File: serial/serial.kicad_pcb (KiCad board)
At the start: 2 copper layers, 24.2 x 12.2 mm, 8 parts, among them J2 Conn_02x03_Odd_Even, Q1 BSS138

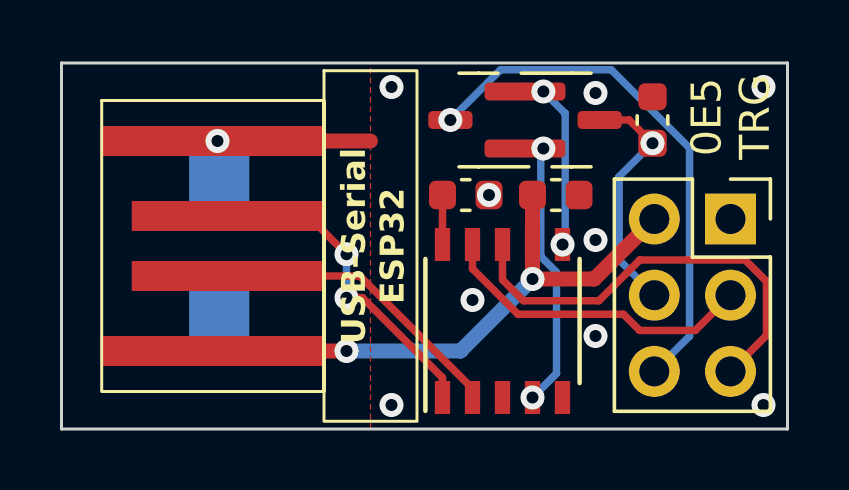
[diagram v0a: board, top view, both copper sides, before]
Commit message: -
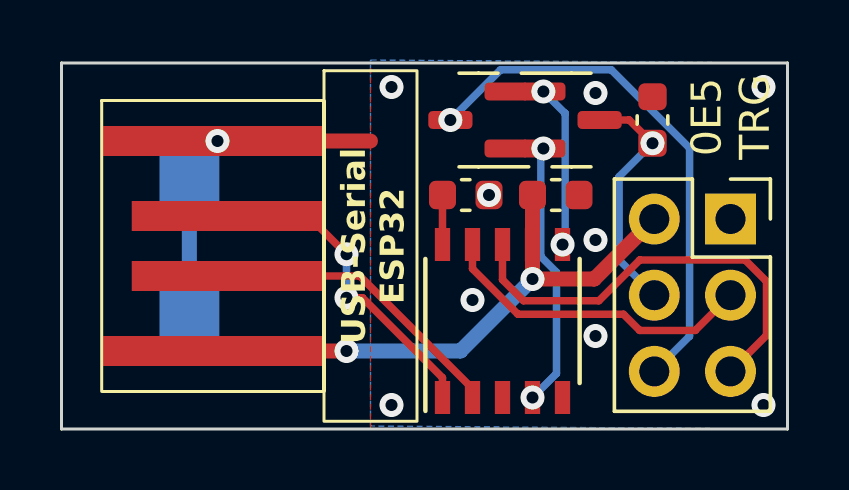
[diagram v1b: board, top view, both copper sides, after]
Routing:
- net Net-(J2-Pin_1): track 5.10 -> 10.6 mm
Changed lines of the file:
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@@
     (pad "4" smd rect (at 4.945 3.5) (size 7.41 1) (layers "F.Cu" "F.Paste" "F.Mask")
       (net 1 "Net-(J2-Pin_2)") (pinfunction "VBUS") (pintype "power_in") (thermal_bridge_angle 45))
-    (pad "5" smd rect (at 5.16 -2.75) (size 2 2.5) (layers "B.Cu" "B.Paste" "B.Mask")
+    (pad "5" smd rect (at 4.16 -2.75) (size 2 2.5) (layers "B.Cu" "B.Paste" "B.Mask")
       (net 2 "Net-(J2-Pin_1)") (pinfunction "SHIELD") (pintype "power_in") (thermal_bridge_angle 45))
-    (pad "6" smd rect (at 5.16 2.75) (size 2 2.5) (layers "B.Cu" "B.Paste" "B.Mask")
+    (pad "6" smd rect (at 4.16 2.75) (size 2 2.5) (layers "B.Cu" "B.Paste" "B.Mask")
       (net 2 "Net-(J2-Pin_1)") (pinfunction "SHIELD") (pintype "power_in") (thermal_bridge_angle 45))
   )
@@
   (via (at 110.9 105.3) (size 0.8) (drill 0.4) (layers "F.Cu" "B.Cu") (free) (net 2))
   (via (at 114.15 98.3) (size 0.8) (drill 0.4) (layers "F.Cu" "B.Cu") (free) (net 2))
+  (segment (start 104.16 97.25) (end 104.16 102.75) (width 0.5) (layer "B.Cu") (net 2))
   (segment (start 112.6 98.3) (end 112.6 99.95) (width 0.25) (layer "F.Cu") (net 3))
   (segment (start 115.113299 102.275) (end 118.633299 102.275) (width 0.25) (layer "F.Cu") (net 4))
@@
     (polygon
       (pts
-        (xy 99.9 93.9)
+        (xy 110.2 93.8)
         (xy 124.1 93.9)
         (xy 124.1 106.1)
-        (xy 99.9 106.1)
+        (xy 110.2 106)
       )
     )
